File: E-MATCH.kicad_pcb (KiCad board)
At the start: 2 copper layers, 20 parts, among them IC1 NCV81071BZR2G, IC2 NCV81071BZR2G, J1 691210910002, J2 691210910002, J3 691210910002, J4 691210910002, Q1 AOSP36326C, Q2 AOSP36326C, Q3 AOSP36326C, Q4 AOSP36326C, U1 TMCS1108A2UQDR

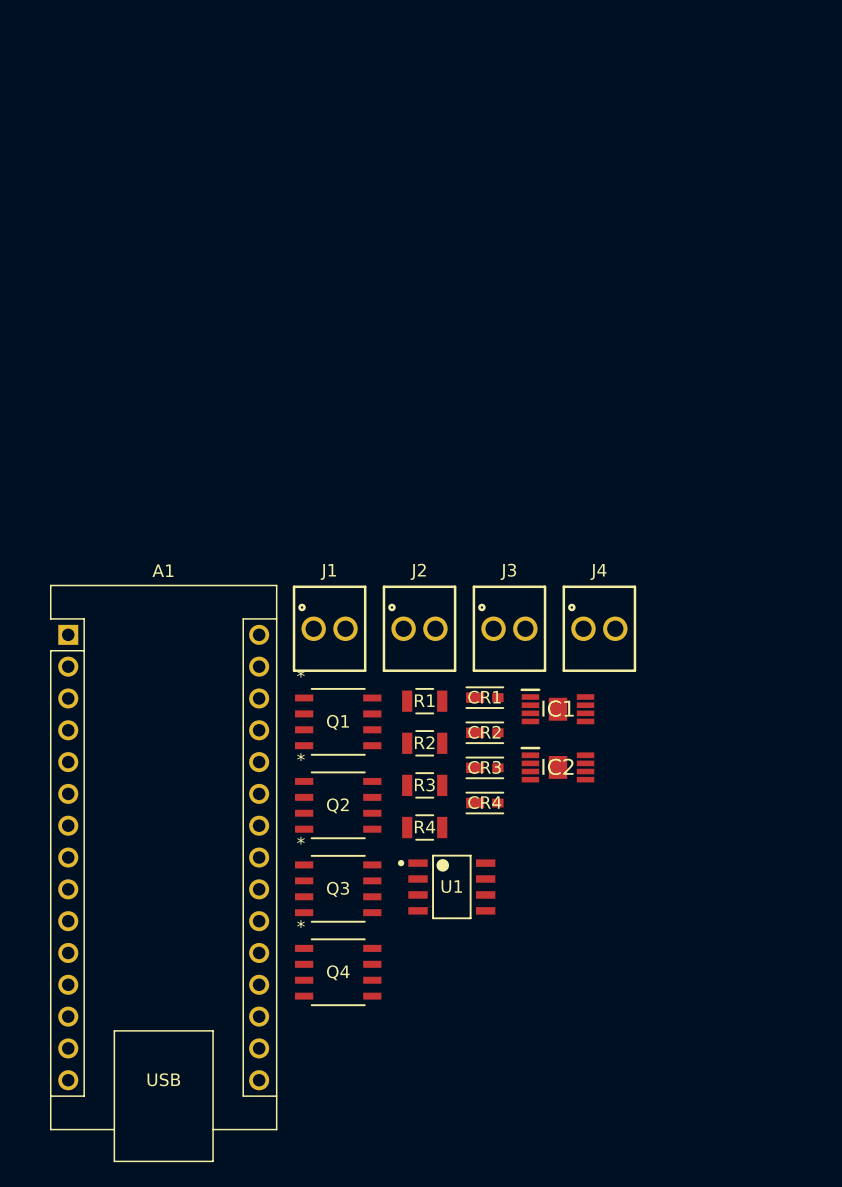
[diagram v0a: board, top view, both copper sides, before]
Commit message: routing
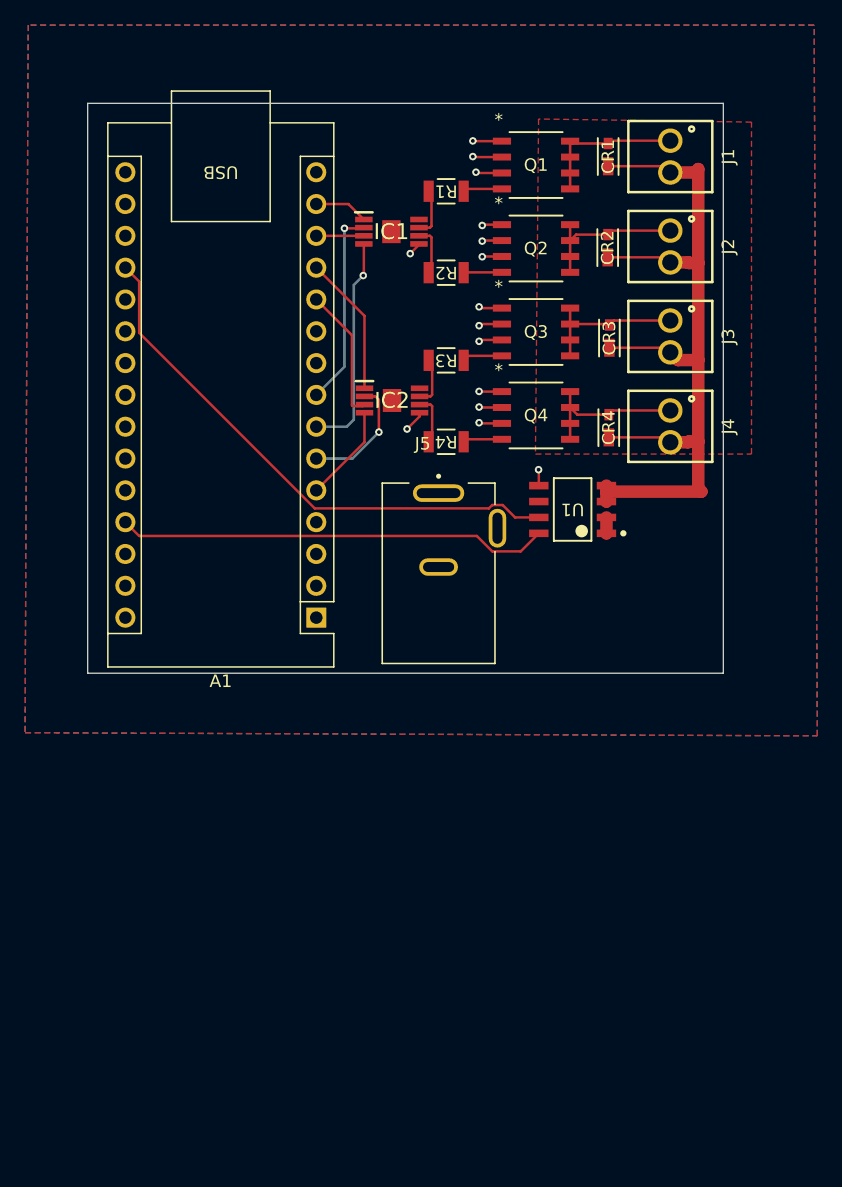
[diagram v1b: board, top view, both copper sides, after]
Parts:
- added J5: DC Jack, DC-Jack:TENSILITY_54-00130, F.Cu at (184.3, 71.0)
- moved Q3 47.2 mm to (192.0, 52.3)
- moved Q4 47.2 mm to (192.0, 58.9)
- moved Q2 47.2 mm to (192.0, 45.6)
- moved Q1 47.2 mm to (192.0, 38.9)
- moved J1 46.5 mm to (202.8, 38.3), turned to -90 degrees
- moved CR1 44.3 mm to (197.8, 38.2), turned to 90 degrees
- moved R1 40.7 mm to (184.9, 41.0), turned to 180 degrees
- moved IC1 40.4 mm to (180.5, 44.2)
- moved CR2 40.0 mm to (197.8, 45.5), turned to 90 degrees
- moved R2 37.6 mm to (184.9, 47.5), turned to 180 degrees
- moved J2 36.5 mm to (202.8, 45.4), turned to -90 degrees
- moved CR3 35.7 mm to (197.9, 52.7), turned to 90 degrees
- moved R3 34.0 mm to (184.9, 54.5), turned to 180 degrees
- moved IC2 32.2 mm to (180.6, 57.7)
- moved U1 31.6 mm to (195.0, 66.4), turned to 180 degrees
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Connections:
- A1 pad 10: Enable_Signal -> unconnected-(A1-D7-Pad10)
- A1 pad 11: unconnected-(A1-D8-Pad11) -> Enable_Signal4
- A1 pad 12: unconnected-(A1-D9-Pad12) -> Enable_Signal3
- A1 pad 13: unconnected-(A1-D10-Pad13) -> Enable_Signal2
- A1 pad 14: unconnected-(A1-D11-Pad14) -> Enable_Signal1
- A1 pad 5: unconnected-(A1-D2-Pad5) -> Trigger_Signal4
- A1 pad 6: unconnected-(A1-D3-Pad6) -> Trigger_Signal3
- A1 pad 7: unconnected-(A1-D4-Pad7) -> Trigger_Signal2
- A1 pad 8: Trigger_Signal -> Trigger_Signal1
- IC1 pad 1: Enable_Signal -> Enable_Signal1
- IC1 pad 2: Trigger_Signal -> Trigger_Signal1
- IC1 pad 3: GND -> Enable_Signal2
- IC1 pad 4: GND -> Trigger_Signal2
- IC2 pad 1: Enable_Signal -> Enable_Signal3
- IC2 pad 2: Trigger_Signal -> Trigger_Signal3
- IC2 pad 3: GND -> Enable_Signal4
- IC2 pad 4: GND -> Trigger_Signal4
- R1 pad 2: unconnected-(R1-Pad2) -> Gate_Drive1
- R2 pad 2: unconnected-(R2-Pad2) -> Gate_Drive2
- R3 pad 2: unconnected-(R3-Pad2) -> Gate_Drive3
- R4 pad 2: unconnected-(R4-Pad2) -> Gate_Drive4
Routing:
- net Net-(CR1-Pad1): track 0.00 -> 64.5 mm
- net Sensor_Output: track 0.00 -> 43.9 mm
- net 5V: track 0.00 -> 34.6 mm
- net GND: track 0.00 -> 26.7 mm, vias 0 -> 15
- net Trigger_Signal2: track 0.00 -> 17.6 mm, vias 0 -> 1
- net Trigger_Signal1: track 0.00 -> 15.8 mm, vias 0 -> 1
- net Net-(CR4-Pad2): track 0.00 -> 12.7 mm
- net Net-(CR2-Pad2): track 0.00 -> 12.1 mm
- net Net-(CR1-Pad2): track 0.00 -> 12.0 mm
- net Net-(CR3-Pad2): track 0.00 -> 12.0 mm
- net Enable_Signal3: track 0.00 -> 11.2 mm
- net Enable_Signal4: track 0.00 -> 10.7 mm
- net Trigger_Signal3: track 0.00 -> 9.71 mm, vias 0 -> 1
- net Trigger_Signal4: track 0.00 -> 7.79 mm
- net Enable_Signal1: track 0.00 -> 4.31 mm
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- added copper zone on B.Cu, net GND
- added copper zone on F.Cu, net Net-(CR1-Pad2)
- added copper zone on F.Cu, net VBAT
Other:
- board outline added: 50.8 x 45.5 mm
